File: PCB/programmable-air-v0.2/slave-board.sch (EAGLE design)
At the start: 26 parts, among them Q1 600mA/40V, Q2 600mA/40V, Q3 600mA/40V

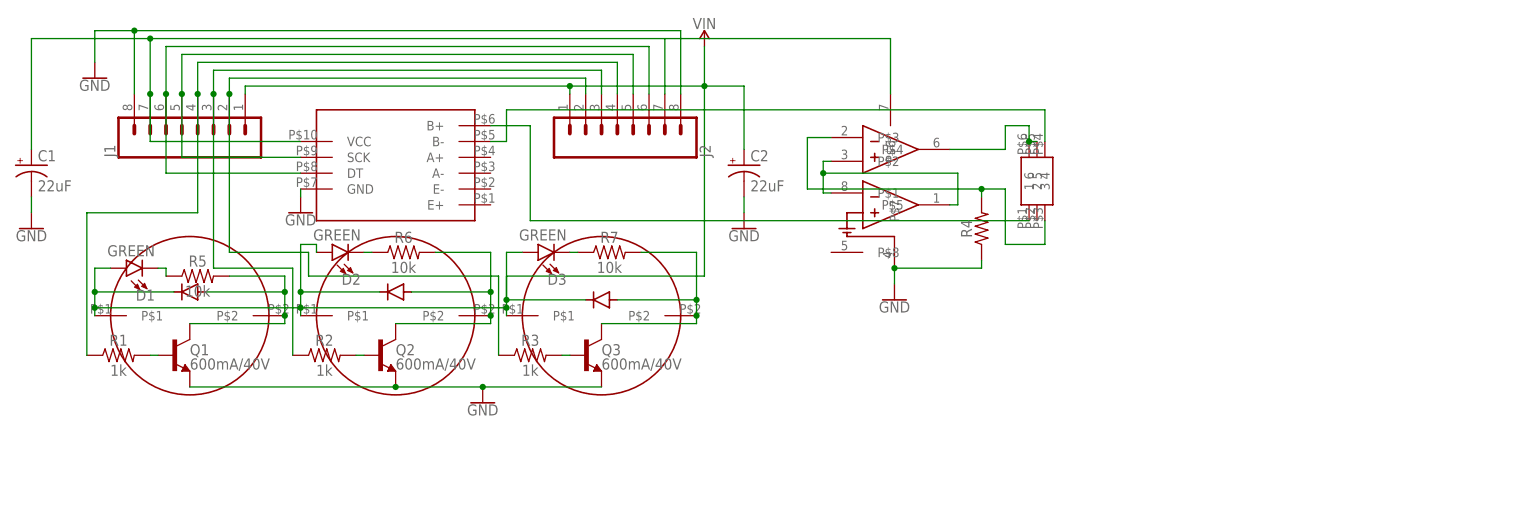
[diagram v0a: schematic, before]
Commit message: LM358 slave board ready
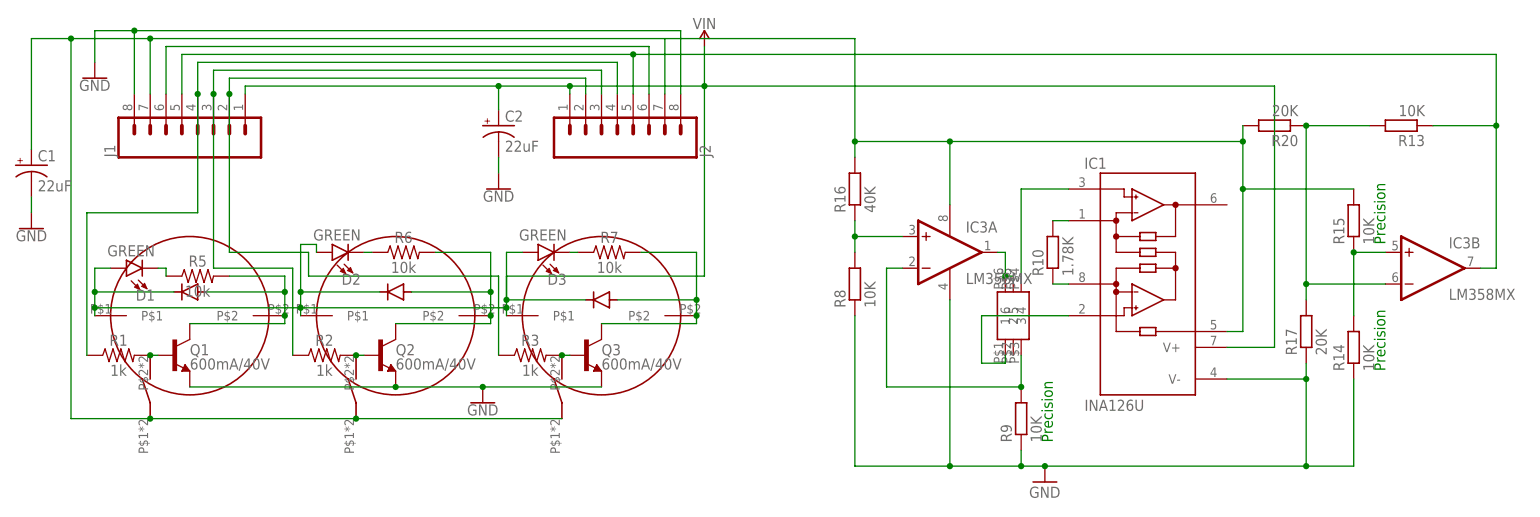
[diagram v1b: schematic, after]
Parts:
- removed R4: (no value), SparkFun-Resistors:RESISTORAXIAL-0.3
- added IC1: INA126U, INA126:INA126U
- added IC3: LM358MX, linear:LM358MX
- added R10: 1.78K, eagle-ltspice:RR0603
- added R13, R14, R15, R8, R9: 10K, eagle-ltspice:RR0603
- added R16: 40K, eagle-ltspice:RR0603
- added R17, R20: 20K, eagle-ltspice:RR0603
- added U$10: BUTTON, programmable-air-components:BUTTON
- U$1: value HX711 -> 2SMPP-03; device programmable-air-components:HX711 -> programmable-air-components:2SMPP-03
- U$8: value 2SMPP-03 -> BUTTON; device programmable-air-components:2SMPP-03 -> programmable-air-components:BUTTON
- U$9: value LM10CN -> BUTTON; device programmable-air-components:LM10CN -> programmable-air-components:BUTTON
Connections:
- removed net N$16: U$8.5, U$8.6, U$9.P$4
- removed net N$17: R4.2, U$8.3, U$9.P$3
- removed net N$21: U$1.B+, U$8.1
- removed net N$22: U$1.B-, U$8.4
- new net N$19: IC3A.OUT, U$1.5, U$1.6
- new net N$20: IC1.+IN, U$1.4
- new net N$24: IC3A.+IN, R16.1, R8.2
- new net N$25: IC1.RG@1, R10.1
- new net N$26: IC1.RG, R10.2
- new net N$27: IC3B.-IN, R13.2, R17.2, R20.1
- new net N$30: IC3B.+IN, R14.2, R15.1
- new net N$31: IC3A.-IN, R9.2, U$1.3
- net GND: now also IC1.V-, IC3P.V-, R14.1, R17.1, R8.1, R9.1; no longer R4.1, U$1.GND, U$9.P$7
- net N$1: now also U$8.P$2
- net N$13: now also IC3B.OUT, R13.1; no longer U$1.SCK
- net N$14: no longer U$1.DT
- net N$15: now also IC1.REF, IC3P.V+, R15.2, R16.2, R20.2, U$10.P$1, U$8.P$1, U$9.P$1; no longer U$1.VCC, U$9.P$6
- net N$2: now also U$9.P$2
- net N$3: now also U$10.P$2
- net N$4: now also IC1.-IN, U$1.1; no longer U$9.P$1, U$9.P$2, U$9.P$5
- net VIN: now also IC1.V+
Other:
- note added: "Precision"
- moved on the sheet: C2
